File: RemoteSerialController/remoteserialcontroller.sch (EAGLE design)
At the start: 46 parts, among them J1 ZX62R-AB-5P, J3 DM3AT-SF-PEJM5, J4 XM3B-0942-132L, Q1 BSS138, Q2 BSS138, U1 ADM3202ARUZ, U2 ESP-WROOM-32, U3 ADP3338AKCZ-3.3, U4 CP2104

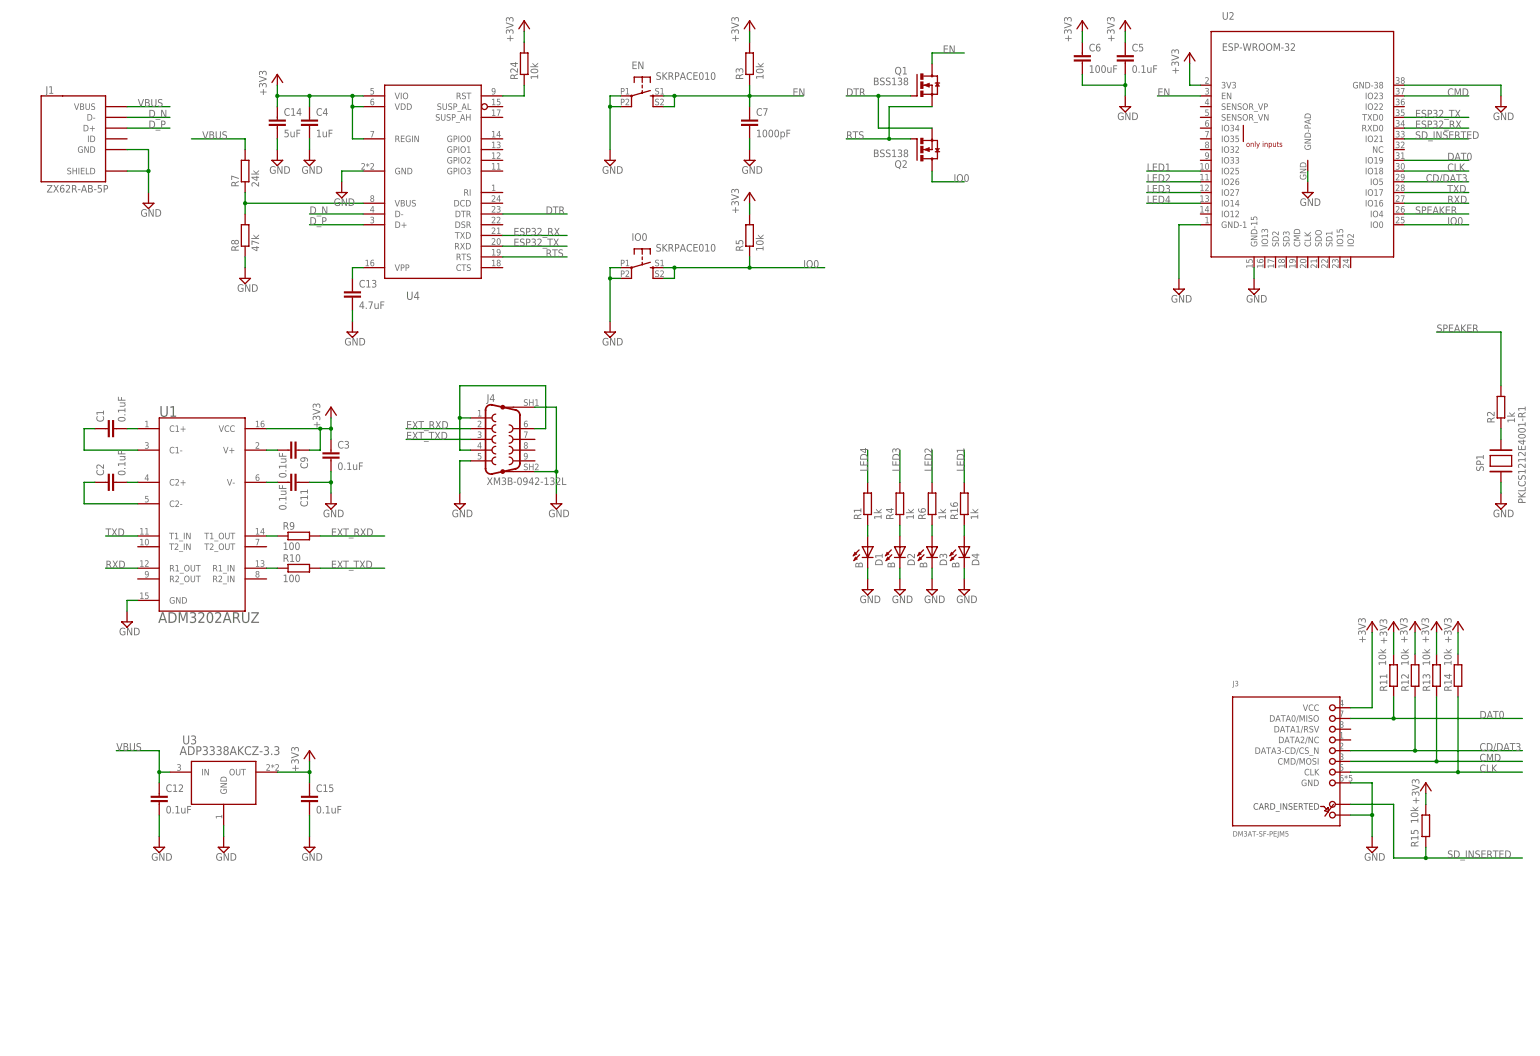
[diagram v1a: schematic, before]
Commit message: [update]update schematic and add BOM
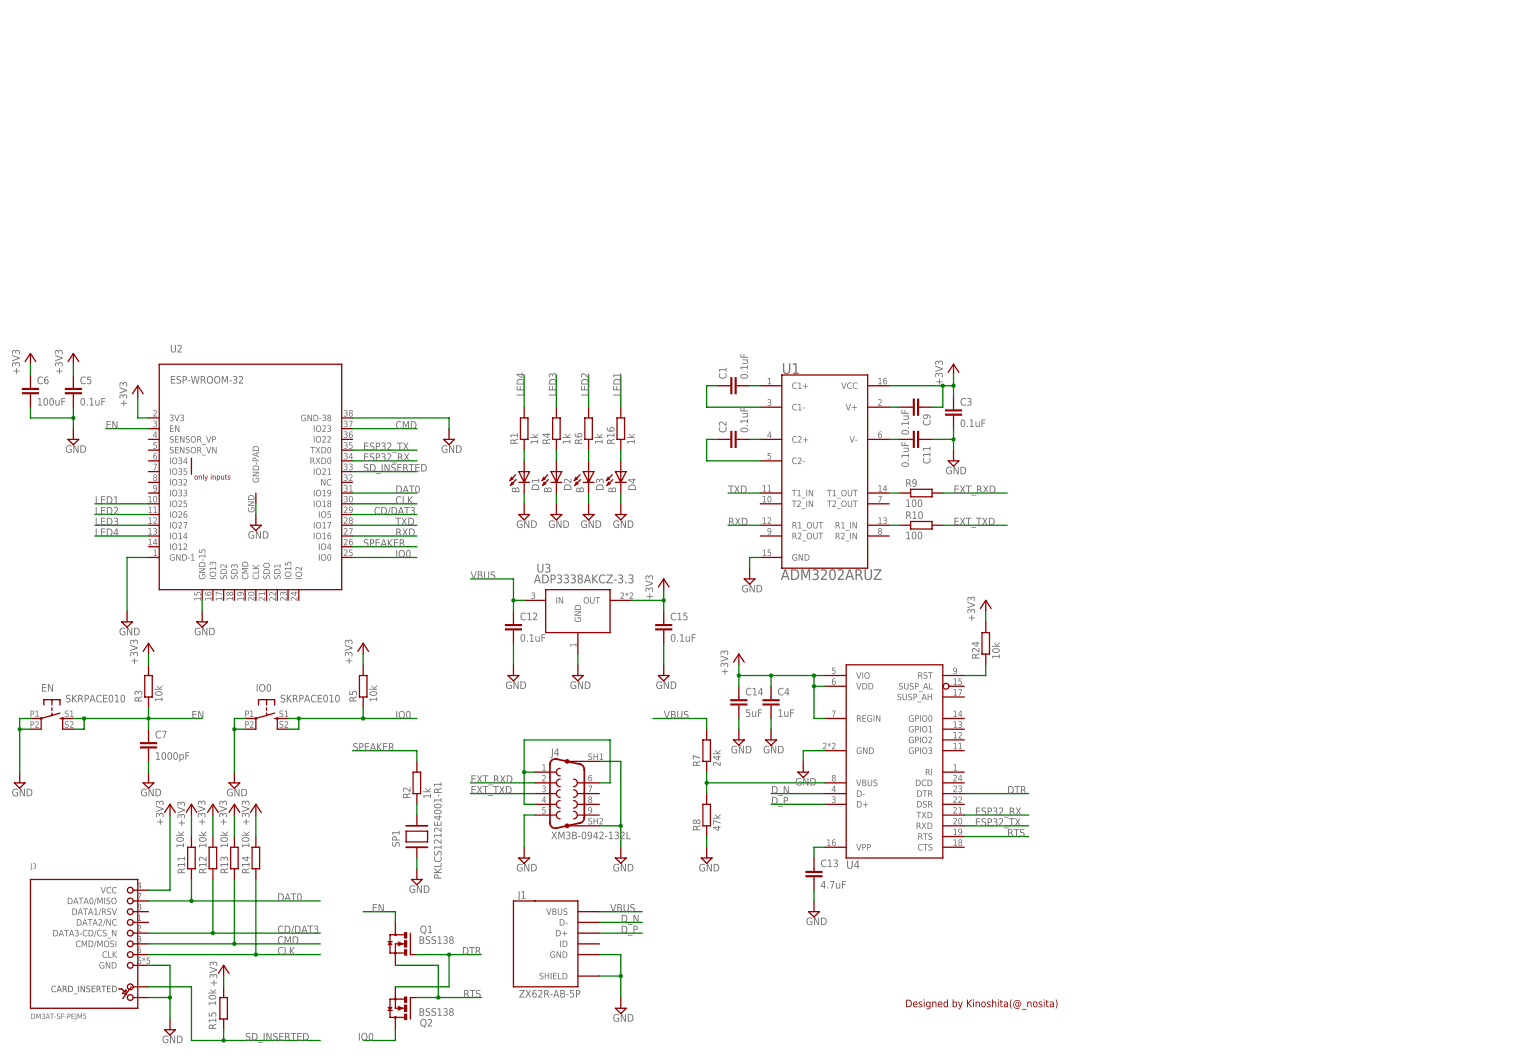
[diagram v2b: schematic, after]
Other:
- note added: "Designed by Kinoshita(@_nosita)"
- moved on the sheet: C1, C11, C12, C13, C14, C15, C2, C3, C4, C5, C6, C7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
